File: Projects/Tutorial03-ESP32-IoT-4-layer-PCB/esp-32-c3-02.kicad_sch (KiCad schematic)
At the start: 0 parts

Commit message: 20260221
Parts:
- added J?: GSD090012SEU, GSD090012SEU:AMPHENOL_GSD090012SEU, symbol GSD090012SEU:GSD090012SEU
- added U2: USBLC6-2SC6, Package_TO_SOT_SMD:SOT-23-6, symbol Power_Protection:USBLC6-2SC6
- added U?: W25Q32JVSSIQ, W25Q32JVSSIQ:SOIC127P790X216-8N, symbol W25Q32JVSSIQ:W25Q32JVSSIQ
- added U?: ESP32-C3-WROOM-02-H4, ESP32-C3-WROOM-02-H4:MODULE_ESP32-C3-WROOM-02-H4, symbol ESP32-C3-WROOM-02-H4:ESP32-C3-WROOM-02-H4
- added U?: CP2102N-Axx-xQFN20, Package_DFN_QFN:SiliconLabs_QFN-20-1EP_3x3mm_P0.5mm, symbol Interface_USB:CP2102N-Axx-xQFN20
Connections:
- new net: U?.19 (GND), U?.20 (GND), U?.21 (GND), U?.22 (GND), U?.23 (GND), U?.24 (GND), U?.25 (GND), U?.26 (GND), U?.27 (GND), U?.28 (GND), U?.29 (GND), U?.30 (GND), U?.31 (GND), U?.32 (GND), U?.33 (GND), U?.34 (GND), U?.35 (GND), U?.36 (GND), U?.37 (GND), U?.38 (GND), U?.39 (GND), U?.9 (GND)
- new net: U?.12 (GND), U?.21 (GND), U?.3 (GND)
- new net: J?.G1 (SHIELD_GND), J?.G2 (SHIELD_GND), J?.G3 (SHIELD_GND), J?.G4 (SHIELD_GND)

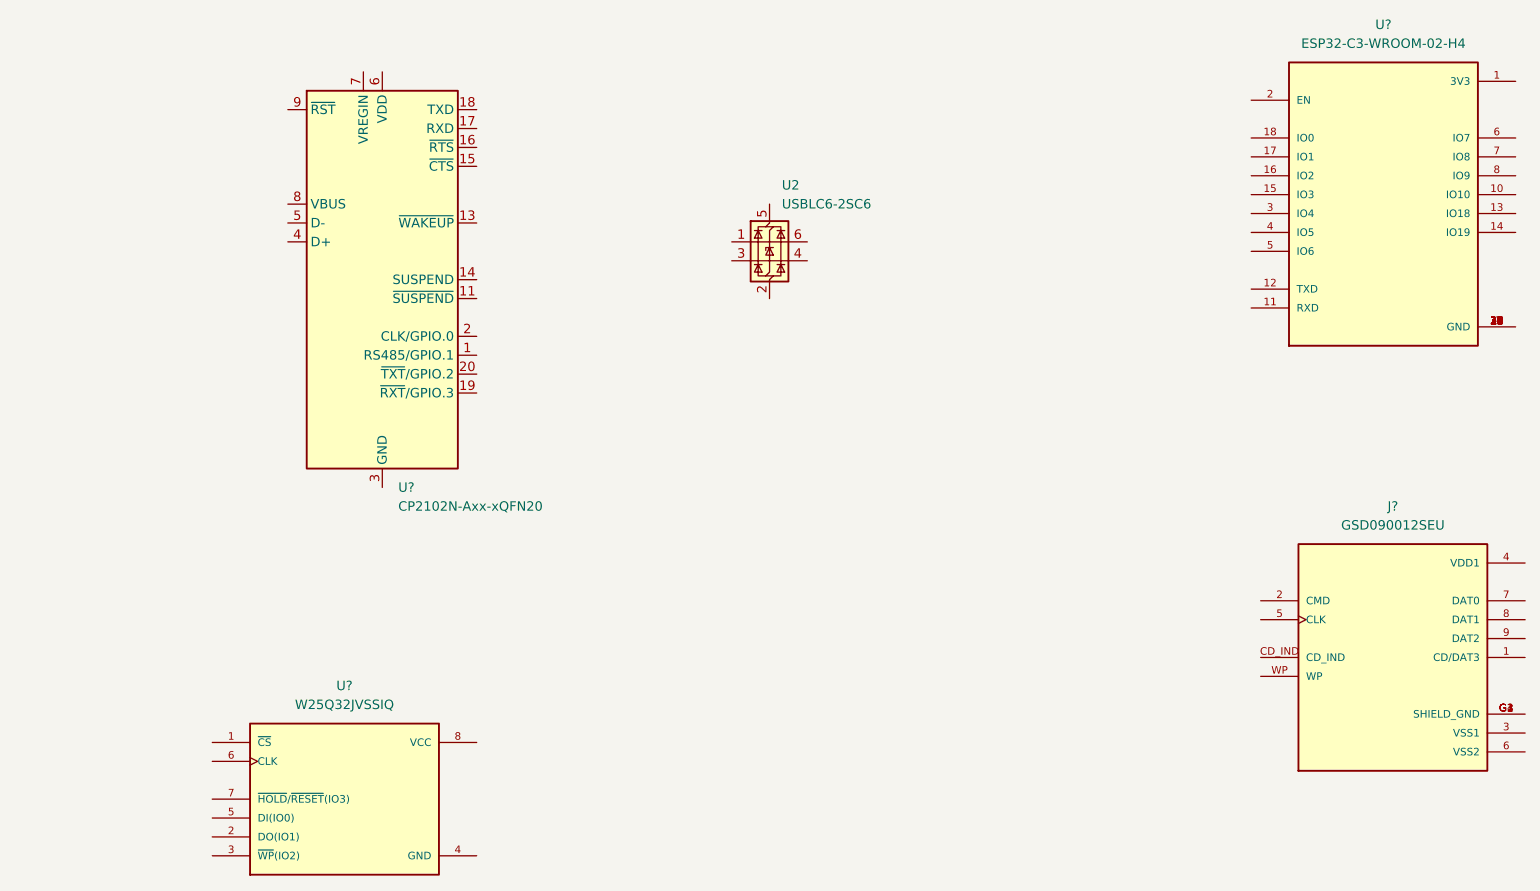
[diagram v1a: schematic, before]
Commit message: 20260221
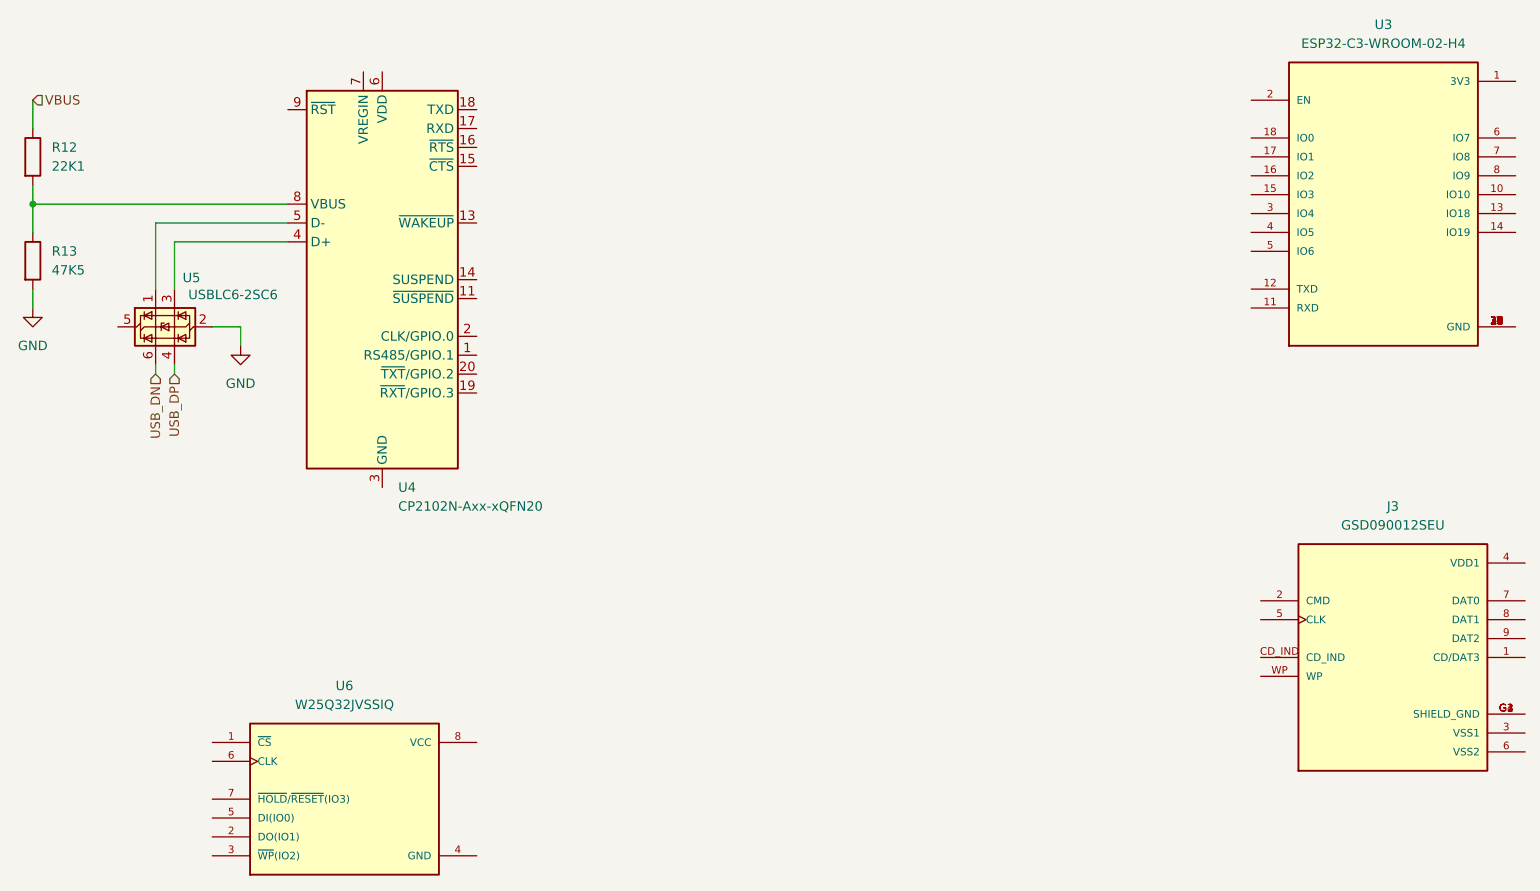
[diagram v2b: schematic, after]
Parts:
- added R12: 22K1, symbol Device:R
- added R13: 47K5, symbol Device:R
- gave numbers to parts that had none: 4
- renumbered U2 to U5
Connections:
- net at U5.1 (I/O1): now also U4.5 (D-)
- net GND: now reaches U5.2 (GND)
- net GND: now also R13.2
- net at U5.3 (I/O2): now also U4.4 (D+)
- net USB_DP: now reaches U5.4 (I/O2)
- net USB_DN: now reaches U5.6 (I/O1)
- net at U4.8 (VBUS): now also R12.2, R13.1
- new net VBUS: R12.1
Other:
- moved on the sheet: U5
